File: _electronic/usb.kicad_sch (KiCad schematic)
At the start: 8 parts

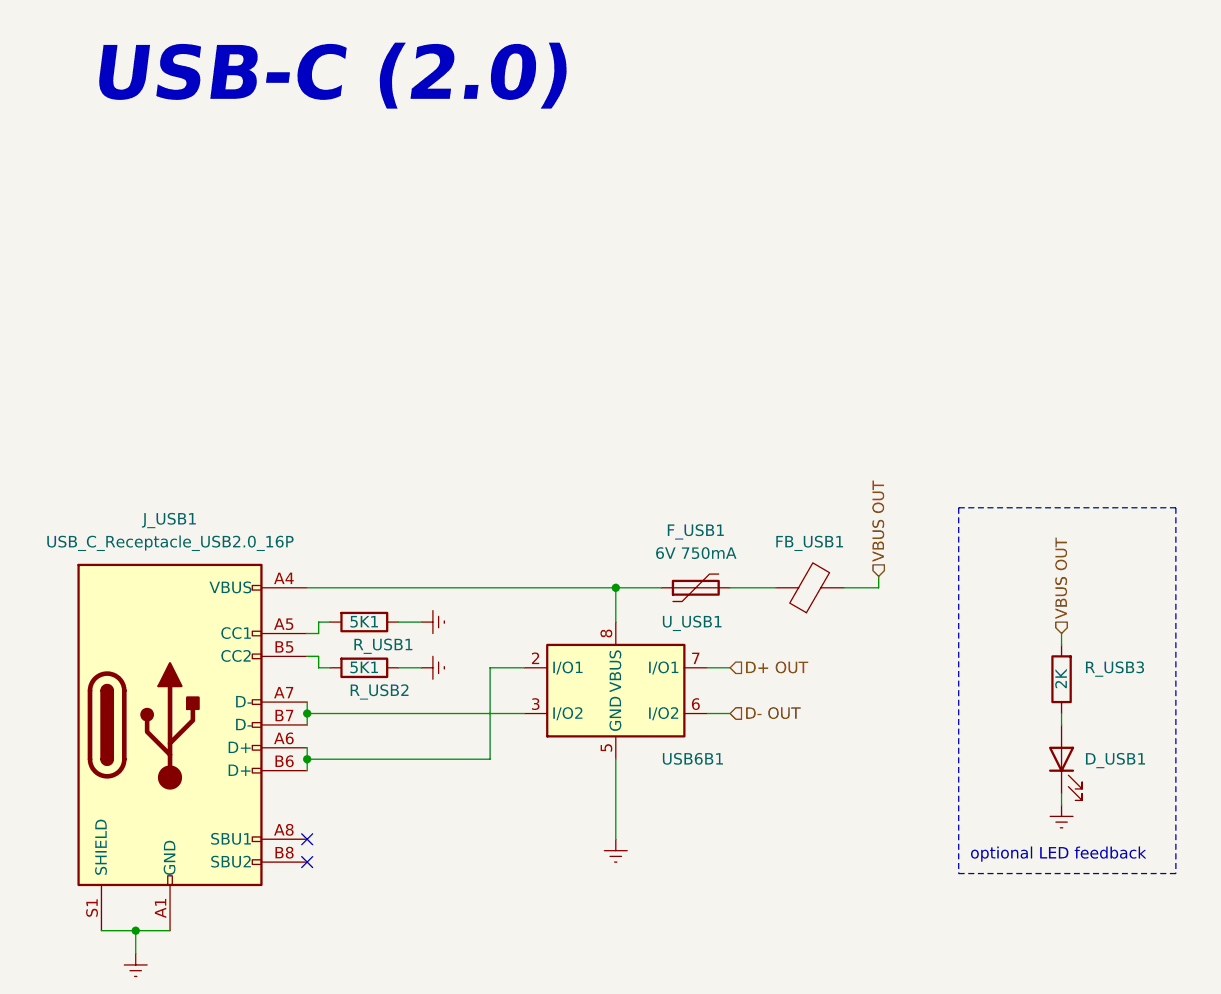
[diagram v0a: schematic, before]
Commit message: sturdyfy E-TKT
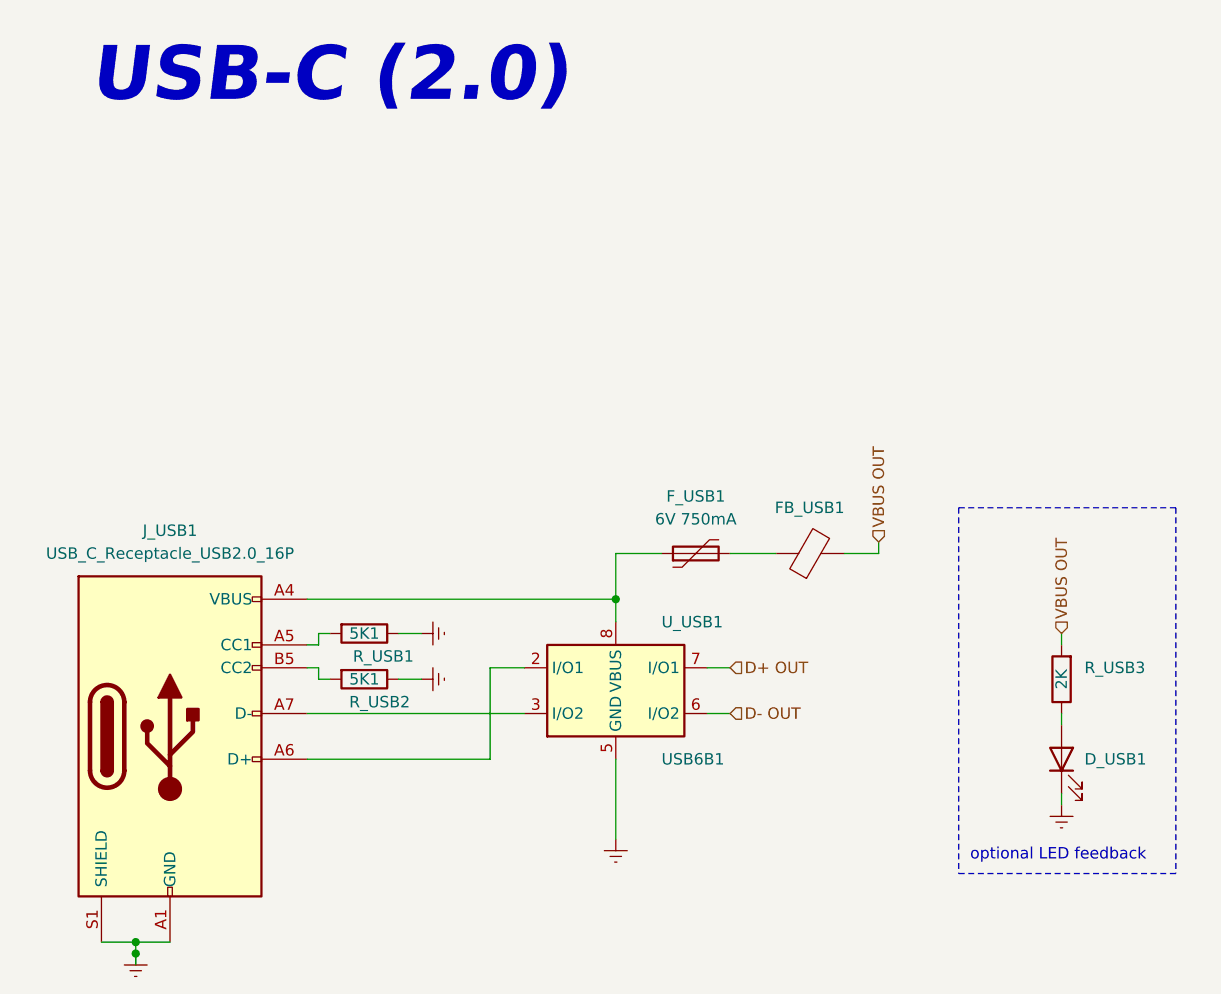
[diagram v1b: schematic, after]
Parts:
- J_USB1: symbol Connector:USB_C_Receptacle_USB2.0_16P -> EASYEDA2KICAD:USB_C_Receptacle_USB2.0_8P
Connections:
- net GNDREF: no longer J_USB1.A12 (GND), J_USB1.B1 (GND), J_USB1.B12 (GND)
- net at F_USB1.1, J_USB1.A4 (VBUS), U_USB1.1 (VBUS)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: no longer J_USB1.A9 (VBUS), J_USB1.B4 (VBUS), J_USB1.B9 (VBUS)
- net at J_USB1.A6 (D+), U_USB1.2 (I/O1): no longer J_USB1.B6 (D+)
- net at J_USB1.A7 (D-), U_USB1.3 (I/O2): no longer J_USB1.B7 (D-)
- no-connect marks 2 -> 0
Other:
- moved on the sheet: FB_USB1, F_USB1, R_USB1, R_USB2
